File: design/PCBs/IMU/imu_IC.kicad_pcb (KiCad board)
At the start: 2 copper layers, 26 x 20 mm, 9 parts, among them J1 Conn_01x04, J2 Conn_01x04, U1 ISM330DHCX

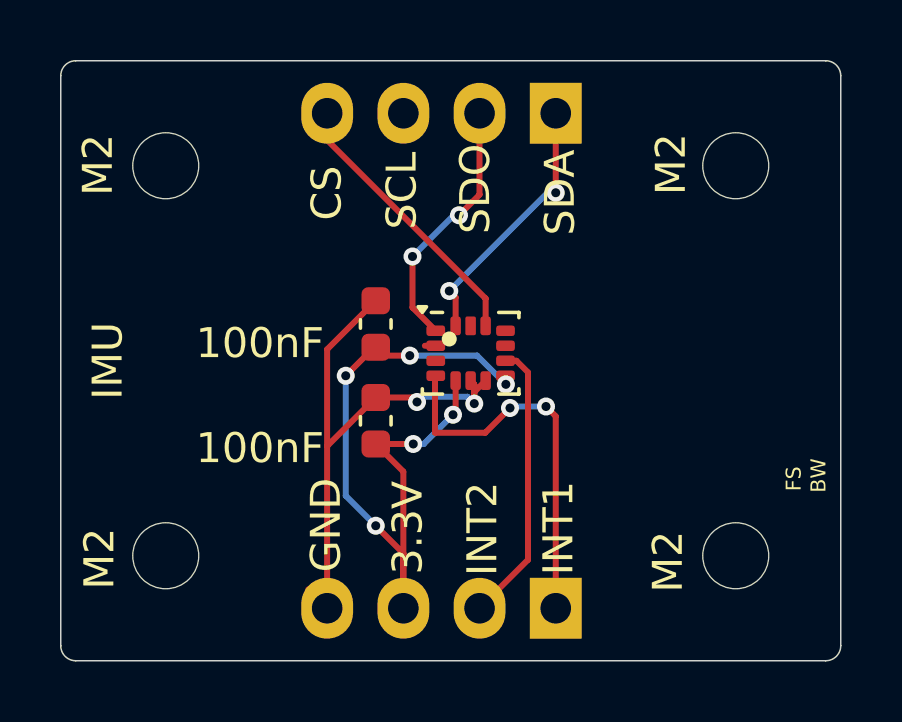
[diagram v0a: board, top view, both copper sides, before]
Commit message: Flywheel 2.1
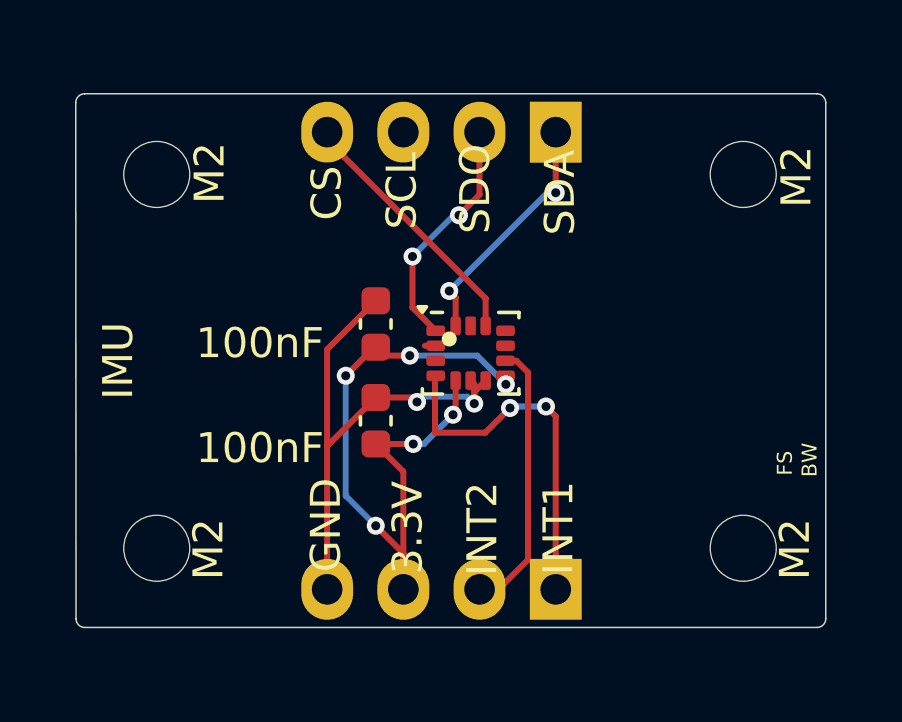
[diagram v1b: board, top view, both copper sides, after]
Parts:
- moved J1 0.63 mm to (141.0, 71.9)
- moved J2 0.63 mm to (141.0, 87.1)
- moved H3 0.42 mm to (127.7, 73.3)
- moved H4 0.39 mm to (127.7, 85.8)
- moved H2 0.38 mm to (147.2, 73.3)
- moved H1 0.35 mm to (147.2, 85.8)
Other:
- board size 26 x 20 mm -> 25 x 17.8 mm
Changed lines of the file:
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@@
 	(footprint "MountingHole:MountingHole_2.2mm_M2"
 		(layer "F.Cu")
-		(at 128 86)
+		(at 127.7 85.75)
 		(descr "Mounting Hole 2.2mm, no annular, M2")
 		(tags "mounting hole 2.2mm no annular m2")
@@
 	(footprint "MountingHole:MountingHole_2.2mm_M2"
 		(layer "F.Cu")
-		(at 147 86)
+		(at 147.25 85.75)
 		(descr "Mounting Hole 2.2mm, no annular, M2")
 		(tags "mounting hole 2.2mm no annular m2")
@@
 	(footprint "Connector:FanPinHeader_1x04_P2.54mm_Vertical"
 		(layer "F.Cu")
-		(at 141 87.75 180)
+		(at 141 87.12 180)
 		(descr "4-pin CPU fan Through hole pin header, e.g. for Wieson part number 2366C888-007 Molex 47053-1000, Foxconn HF27040-M1, Tyco 1470947-1 or equivalent, see http://www.formfactors.org/developer%5Cspecs%5Crev1_2_public.pdf")
 		(tags "pin header 4-pin CPU fan")
@@
 	(footprint "Connector:FanPinHeader_1x04_P2.54mm_Vertical"
 		(layer "F.Cu")
-		(at 141 71.25 180)
+		(at 141 71.88 180)
 		(descr "4-pin CPU fan Through hole pin header, e.g. for Wieson part number 2366C888-007 Molex 47053-1000, Foxconn HF27040-M1, Tyco 1470947-1 or equivalent, see http://www.formfactors.org/developer%5Cspecs%5Crev1_2_public.pdf")
 		(tags "pin header 4-pin CPU fan")
@@
 	(footprint "MountingHole:MountingHole_2.2mm_M2"
 		(layer "F.Cu")
-		(at 147 73)
+		(at 147.25 73.29)
 		(descr "Mounting Hole 2.2mm, no annular, M2")
 		(tags "mounting hole 2.2mm no annular m2")
@@
 	(footprint "MountingHole:MountingHole_2.2mm_M2"
 		(layer "F.Cu")
-		(at 128 73)
+		(at 127.7 73.29)
 		(descr "Mounting Hole 2.2mm, no annular, M2")
 		(tags "mounting hole 2.2mm no annular m2")
@@
 		(layer "F.SilkS")
 	)
-	(gr_line
-		(start 124.5 89)
-		(end 124.5 70)
+	(gr_arc
+		(start 125 70.9)
+		(mid 125.087868 70.687868)
+		(end 125.3 70.6)
 		(stroke
 			(width 0.05)
@@
 	)
 	(gr_arc
-		(start 150.5 89)
-		(mid 150.353553 89.353553)
-		(end 150 89.5)
+		(start 125.31 88.39)
+		(mid 125.098384 88.308688)
+		(end 125.009828 88.1)
 		(stroke
 			(width 0.05)
@@
 	)
 	(gr_line
-		(start 125 69.5)
-		(end 150 69.5)
+		(start 150 88.1)
+		(end 150 70.9)
 		(stroke
 			(width 0.05)
@@
 	)
 	(gr_arc
-		(start 150 69.5)
-		(mid 150.353553 69.646447)
-		(end 150.5 70)
+		(start 150 88.1)
+		(mid 149.915061 88.305061)
+		(end 149.71 88.39)
 		(stroke
 			(width 0.05)
@@
 	)
 	(gr_line
-		(start 150 89.5)
-		(end 125 89.5)
+		(start 125.31 88.39)
+		(end 149.71 88.39)
 		(stroke
 			(width 0.05)
@@
 	)
 	(gr_arc
-		(start 124.5 70)
-		(mid 124.646447 69.646447)
-		(end 125 69.5)
+		(start 149.7 70.6)
+		(mid 149.912132 70.687868)
+		(end 150 70.9)
 		(stroke
 			(width 0.05)
@@
 		(layer "Edge.Cuts")
 	)
-	(gr_arc
-		(start 125 89.5)
-		(mid 124.646447 89.353553)
-		(end 124.5 89)
+	(gr_line
+		(start 149.7 70.6)
+		(end 125.3 70.6)
 		(stroke
 			(width 0.05)
@@
 	)
 	(gr_line
-		(start 150.5 70)
-		(end 150.5 89)
+		(start 125.009828 88.1)
+		(end 125 70.9)
 		(stroke
 			(width 0.05)
@@
 	)
 	(gr_text "CUBITRON"
-		(at 126.625 76.05 90)
+		(at 126.975 76.05 90)
 		(layer "B.SilkS" knockout)
 		(effects
@@
 	)
 	(gr_text "BW"
-		(at 150.05 83.9 90)
+		(at 149.755 83.38 90)
 		(layer "F.SilkS")
 		(effects
@@
 	)
 	(gr_text "IMU\n"
-		(at 126.65 80.8 90)
+		(at 127 80.8 90)
 		(layer "F.SilkS" knockout)
 		(effects
@@
 	)
 	(gr_text "M2"
-		(at 145.325 87.225 90)
+		(at 149.56 86.81 90)
 		(layer "F.SilkS")
 		(effects
@@
 	)
 	(gr_text "M2"
-		(at 145.425 73.975 90)
+		(at 149.61 74.4 90)
 		(layer "F.SilkS")
 		(effects
@@
 	)
 	(gr_text "M2"
-		(at 126.325 74 90)
+		(at 130.05 74.27 90)
 		(layer "F.SilkS")
 		(effects
@@
 	)
 	(gr_text "M2"
-		(at 126.375 87.125 90)
+		(at 130.01 86.81 90)
 		(layer "F.SilkS")
 		(effects
@@
 	)
 	(gr_text "FS"
-		(at 149.225 83.85 90)
+		(at 148.93 83.33 90)
 		(layer "F.SilkS")
 		(effects
